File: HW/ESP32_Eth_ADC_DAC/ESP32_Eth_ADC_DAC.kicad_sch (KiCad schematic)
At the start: 6 parts, among them J1 2.54mm female 90deg, U1 ESP32-ETH01, U2 PCM5102A_dac, U3 WM8782S_adc

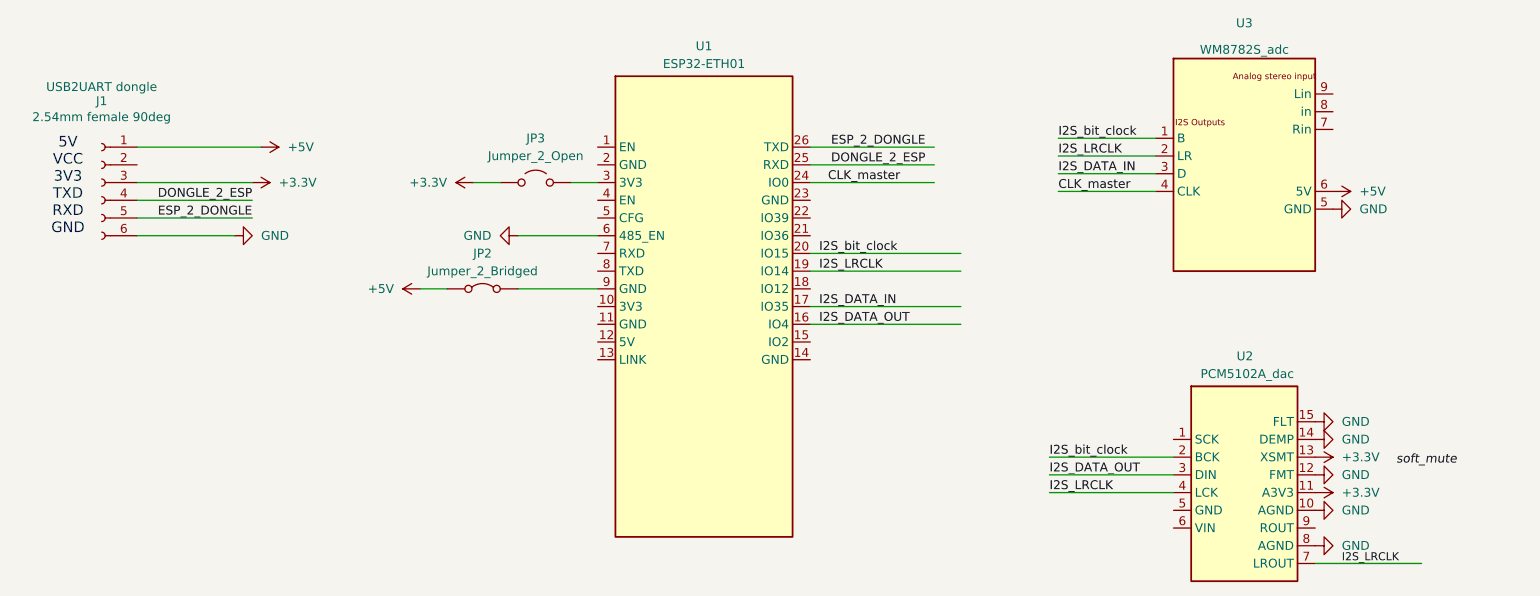
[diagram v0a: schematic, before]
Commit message: Git fixed
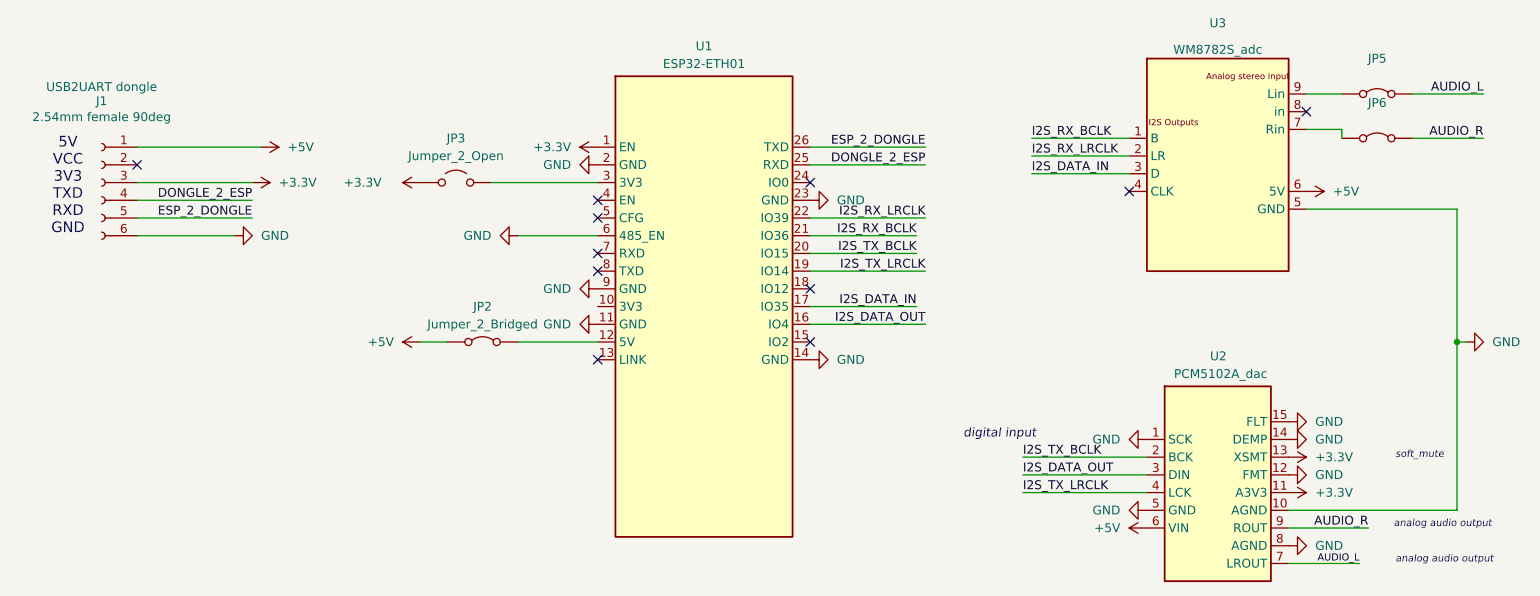
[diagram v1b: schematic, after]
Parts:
- added JP5, JP6: Jumper_2_Bridged, symbol Jumper:Jumper_2_Bridged
- U2: footprint ESP32_Eth_ADC_DAC:PCM5102A_dac -> Package_SO:TSSOP-20_4.4x6.5mm_P0.65mm
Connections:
- net +3.3V: now also U1.1 (EN)
- net +5V: now also U2.6 (VIN)
- net GND: now also U1.11 (GND), U1.14 (GND), U1.2 (GND), U1.23 (GND), U1.9 (GND), U2.1 (SCK), U2.5 (GND)
- net at U3.7 (Rin): now also JP6.1 (A)
- net at U3.9 (Lin): now also JP5.1 (A)
- net at U1.12 (5V): now also JP2.2 (B)
- net I2S_RX_BCLK: now reaches U1.21 (IO36)
- net I2S_RX_BCLK: now also U3.1 (B)
- net I2S_RX_LRCLK: now reaches U1.22 (IO39)
- net I2S_RX_LRCLK: now also U3.2 (LR)
- net AUDIO_R: now reaches U2.9 (ROUT)
- net AUDIO_R: now also JP6.2 (B)
- net CLK_master: no longer names the net of U3.4 (CLK)
- net CLK_master: no longer U1.24 (IO0)
- net I2S_LRCLK renamed I2S_TX_LRCLK
- net I2S_TX_LRCLK: no longer U2.7 (LROUT), U3.2 (LR)
- net I2S_bit_clock renamed I2S_TX_BCLK
- net I2S_TX_BCLK: no longer U3.1 (B)
- new net AUDIO_L: JP5.2 (B), U2.7 (LROUT)
- no-connect marks 0 -> 11
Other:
- note added: "analog audio output"
- note added: "digital input"
- note added: "soft_mute"
- moved on the sheet: JP2, JP3, U2, U3
